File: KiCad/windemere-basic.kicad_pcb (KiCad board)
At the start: 2 copper layers, 152.4 x 158.7 mm, 65 parts, among them J2 Barrel_Jack, J3 Connector, SW1 Reset Button, U1 L7805, U2 74HC00, U3 WD65C02, U4 28C256, U5 62256, U6 WD65C22, U7 MM74C922, U8 HD44780U, U9 MCP102-475, X1 1MHz

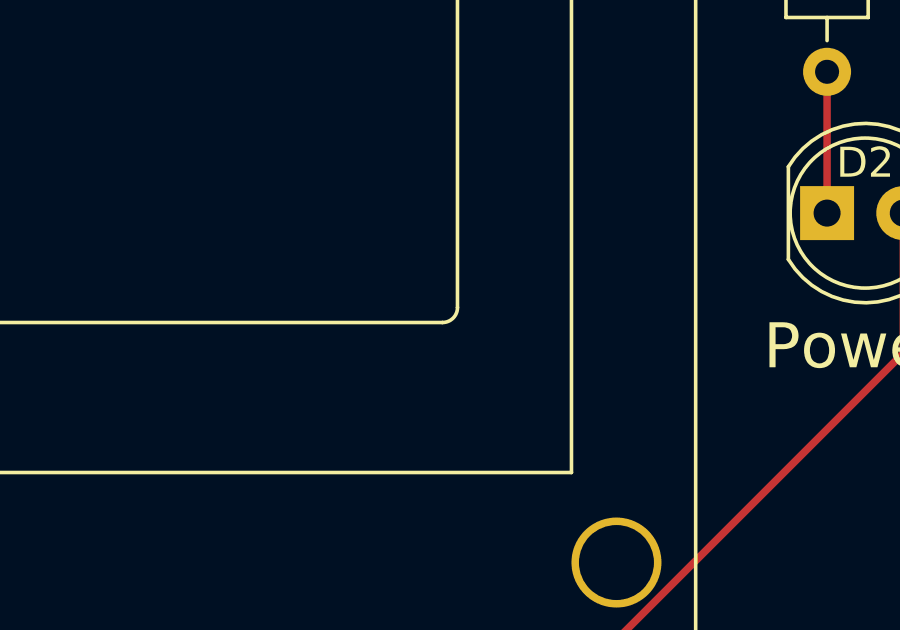
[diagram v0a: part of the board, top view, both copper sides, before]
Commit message: Cleanup the Schematic
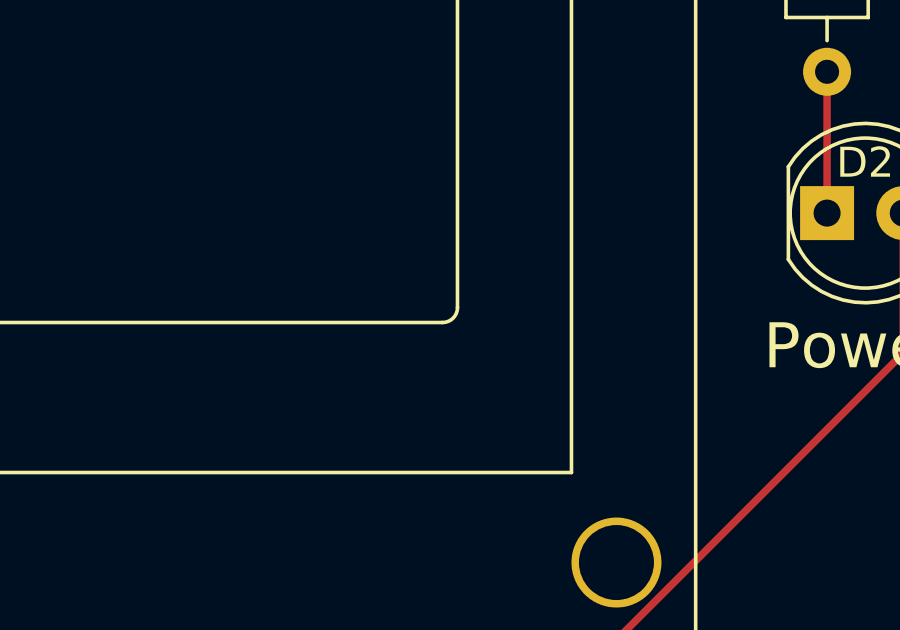
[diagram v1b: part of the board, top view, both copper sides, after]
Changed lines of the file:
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@@
     (fp_arc (start 63.7 8) (mid 64.053553 8.146447) (end 64.2 8.5) (layer "F.SilkS") (width 0.12))
     (fp_arc (start 0.20066 22.9997) (mid -0.153162 22.853142) (end -0.29972 22.49932) (layer "F.SilkS") (width 0.12))
-    (fp_arc (start 64.20104 22.49932) (mid 64.054479 22.85315) (end 63.70066 22.9997) (layer "F.SilkS") (width 0.12))
+    (fp_arc (start 64.20104 22.49932) (mid 64.054473 22.853115) (end 63.70066 22.9997) (layer "F.SilkS") (width 0.12))
     (fp_line (start -8.25 33.75) (end 72.25 33.75) (layer "F.CrtYd") (width 0.05))
     (fp_line (start 72.25 -2.75) (end 72.25 33.75) (layer "F.CrtYd") (width 0.05))
